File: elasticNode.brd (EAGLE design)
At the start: 58.2 x 52.5 mm, 113 parts, among them J1 ISP_CONN_6PIN, J10 ISP_CONN_6PIN, J2 FEMALE_HEADER_2X2, J3 FEMALE_HEADER_2X1, J4 FEMALE_HEADER_2X1, J5 FEMALE_HEADER_10X2, J8 USB_CONNSMT, J9 USB_CONNSMT, U1 ATMEGA64AQFN, U10 LTC3419DFN, U11 ATMEGA32U4, U2 SST26VF032B, U3 MRF24J40MA, U4 SPARTAN6-LX9, U5 SST26VF032B, U6 PAC1720, U7 PAC1720, U8 PAC1720, U9 FT232RSSOP28, X1 12MHz, X2 50MHz, X3 32MHz, X4 12MHz

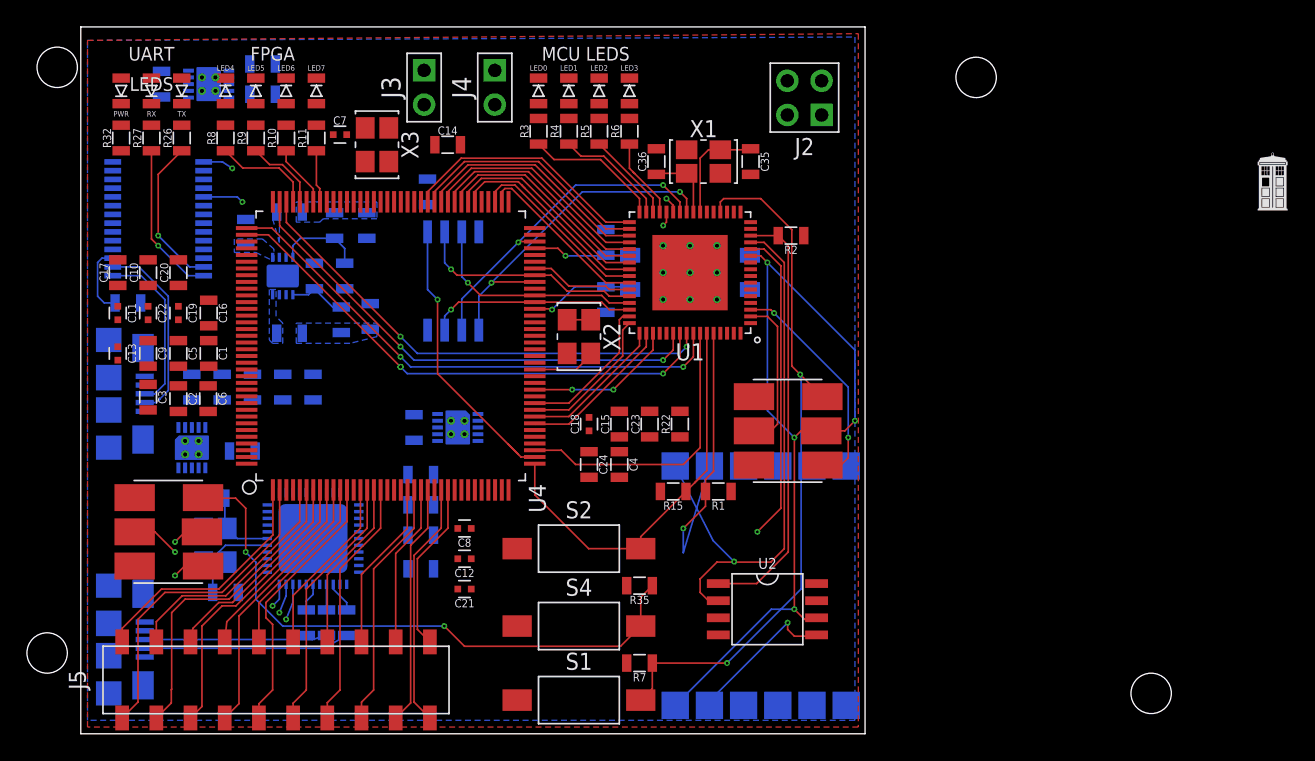
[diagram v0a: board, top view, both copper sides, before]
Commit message: New layout is done
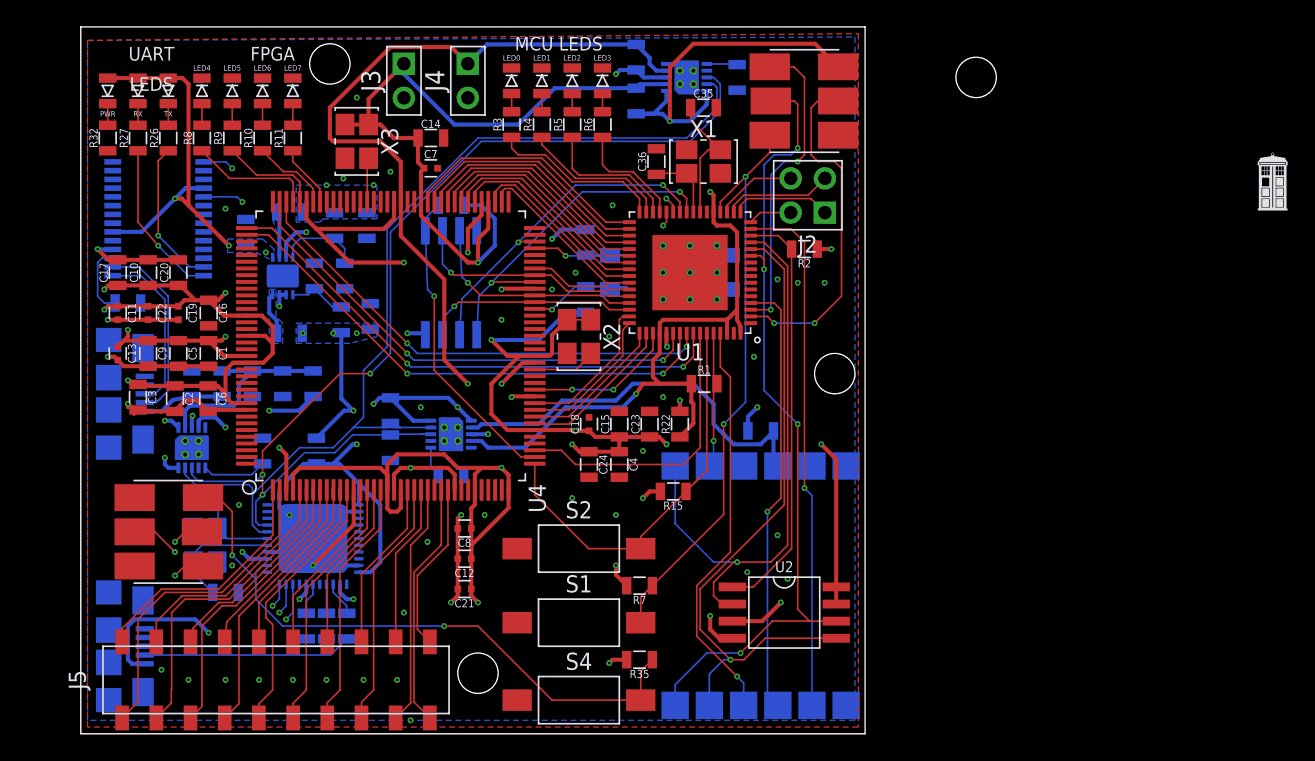
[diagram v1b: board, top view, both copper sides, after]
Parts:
- moved R21 42.8 mm to (48.8, 48.8), turned to 90 degrees
- moved U7 35.5 mm to (45.0, 48.8), turned to 180 degrees
- moved R17 27.9 mm to (41.2, 50.2), turned to 270 degrees
- moved R19 27.9 mm to (41.2, 47.0), turned to 270 degrees
- moved R36 25.8 mm to (50.5, 22.5), turned to 180 degrees
- moved J1 24.5 mm to (53.8, 47.0), turned to 270 degrees
- moved R24 9.52 mm to (23.0, 24.0), turned to 90 degrees
- moved R25 9.28 mm to (23.0, 21.2), turned to 90 degrees
- moved R1 8.07 mm to (46.3, 26.0), turned to 0 degrees
- moved R16 7.95 mm to (17.5, 21.0), turned to 90 degrees
- moved J2 7.25 mm to (54.0, 40.0)
- moved C7 7.20 mm to (26.0, 42.0)
- moved R7 5.75 mm to (41.5, 11.0)
- moved S1 5.75 mm to (37.0, 8.25)
- moved R35 5.50 mm to (41.5, 5.50)
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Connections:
- removed net N$33: U1.15
- net 3V3: no longer R25.2
- net GND: now also U11.45
- net MCU_GPIO_0: now also J2.1, U1.17; no longer J2.4, U1.16
- net MCU_GPIO_1: now also J2.2, U1.18; no longer J2.3, U1.6
- net MCU_GPIO_2: now also J2.3, U1.19; no longer J2.2, U1.17
- net MCU_GPIO_3: now also J2.4, U1.16; no longer J2.1, U1.61
- net MCU_LED1: no longer U1.10
- net MCU_LED2: no longer U1.4
- net MCU_LED3: no longer U1.5
- net SDA: now also R25.2; no longer R25.1
- net WIRELESS_INT: now also U1.61; no longer U1.9
- net WIRELESS_RESET: now also U1.15; no longer U1.7
- net WIRELESS_WAKE: now also U1.4; no longer U1.8
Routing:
- net FPGA_VCCAUX: track 1.75 -> 265.9 mm, vias 0 -> 16
- net 3V3: track 0.00 -> 134.6 mm, vias 0 -> 13
- net FPGA_VCCINT: track 0.00 -> 109.3 mm, vias 0 -> 5
- net SDA: track 0.00 -> 81.4 mm, vias 0 -> 3
- net MON_VCC: track 0.00 -> 76.8 mm, vias 0 -> 4
- net GND: track 0.00 -> 76.0 mm, vias 0 -> 48
- net SCL: track 0.00 -> 73.2 mm
- net MCU_VCC: track 0.00 -> 66.5 mm, vias 0 -> 6
- net 5V: track 0.00 -> 63.0 mm, vias 0 -> 6
- net WIRELESS_RESET: track 0.00 -> 39.0 mm, vias 0 -> 1
- net WIRELESS_WAKE: track 0.00 -> 32.6 mm, vias 0 -> 1
- net WIRELESS_INT: track 0.00 -> 30.4 mm, vias 0 -> 1
- net WIRELESS_VCC: track 0.00 -> 29.7 mm
- net 1V2: track 0.00 -> 28.3 mm, vias 0 -> 3
- net USB2_VCC: track 0.00 -> 26.3 mm, vias 0 -> 3
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- added copper zone on layer 3, net FPGA_VCCAUX
- added copper zone on layer 3, net MCU_VCC
- removed copper zone on layer 3, net 3V3
